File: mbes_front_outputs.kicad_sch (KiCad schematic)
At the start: 41 parts, among them IC1 BDX34C, IC2 BDX34C, IC3 BDX34C, IC4 BDX34C, Q1 D45VH10, Q10 BC337, Q2 D45VH10, Q3 BC337, Q4 BC337, Q5 BC337, Q6 BC337, Q7 BC337, Q8 BC337, Q9 BC337

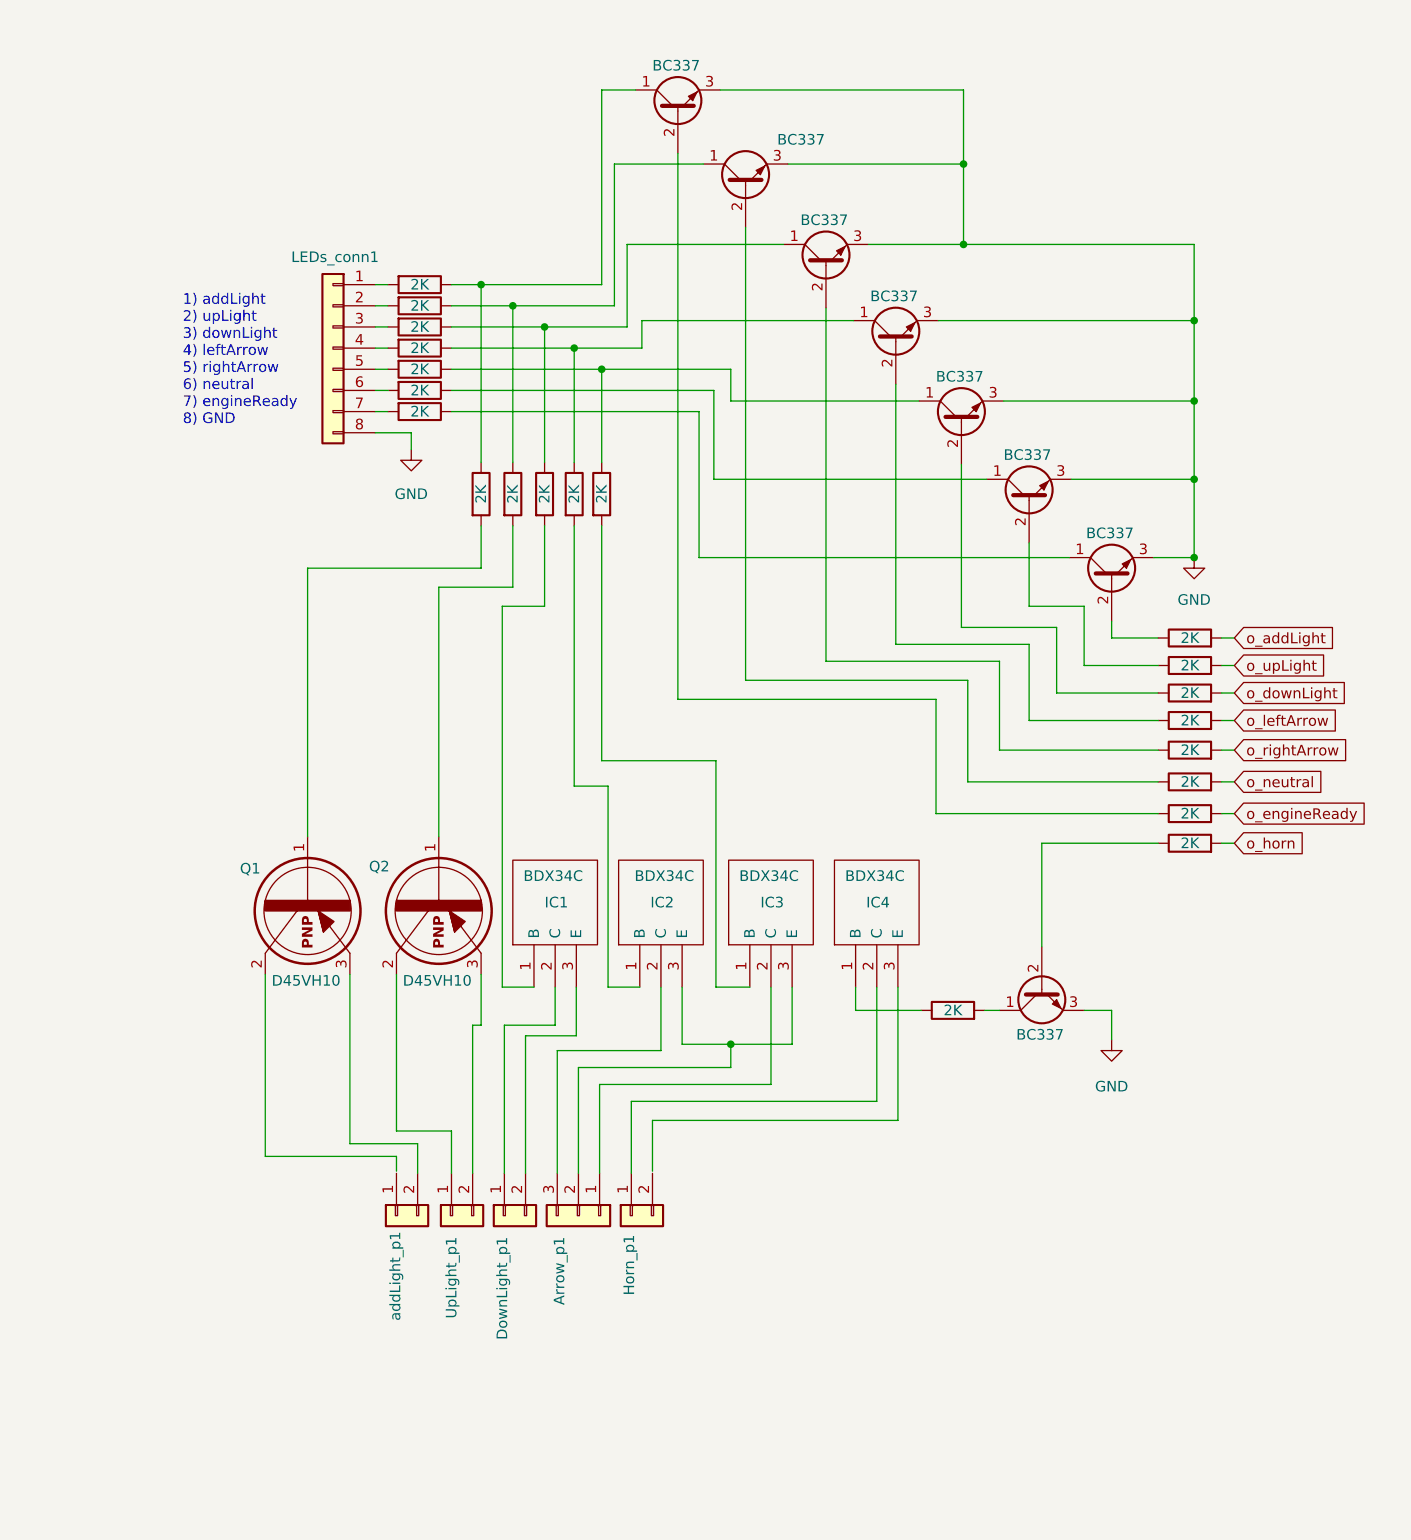
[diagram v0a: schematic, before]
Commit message: First release of all-in-one solution
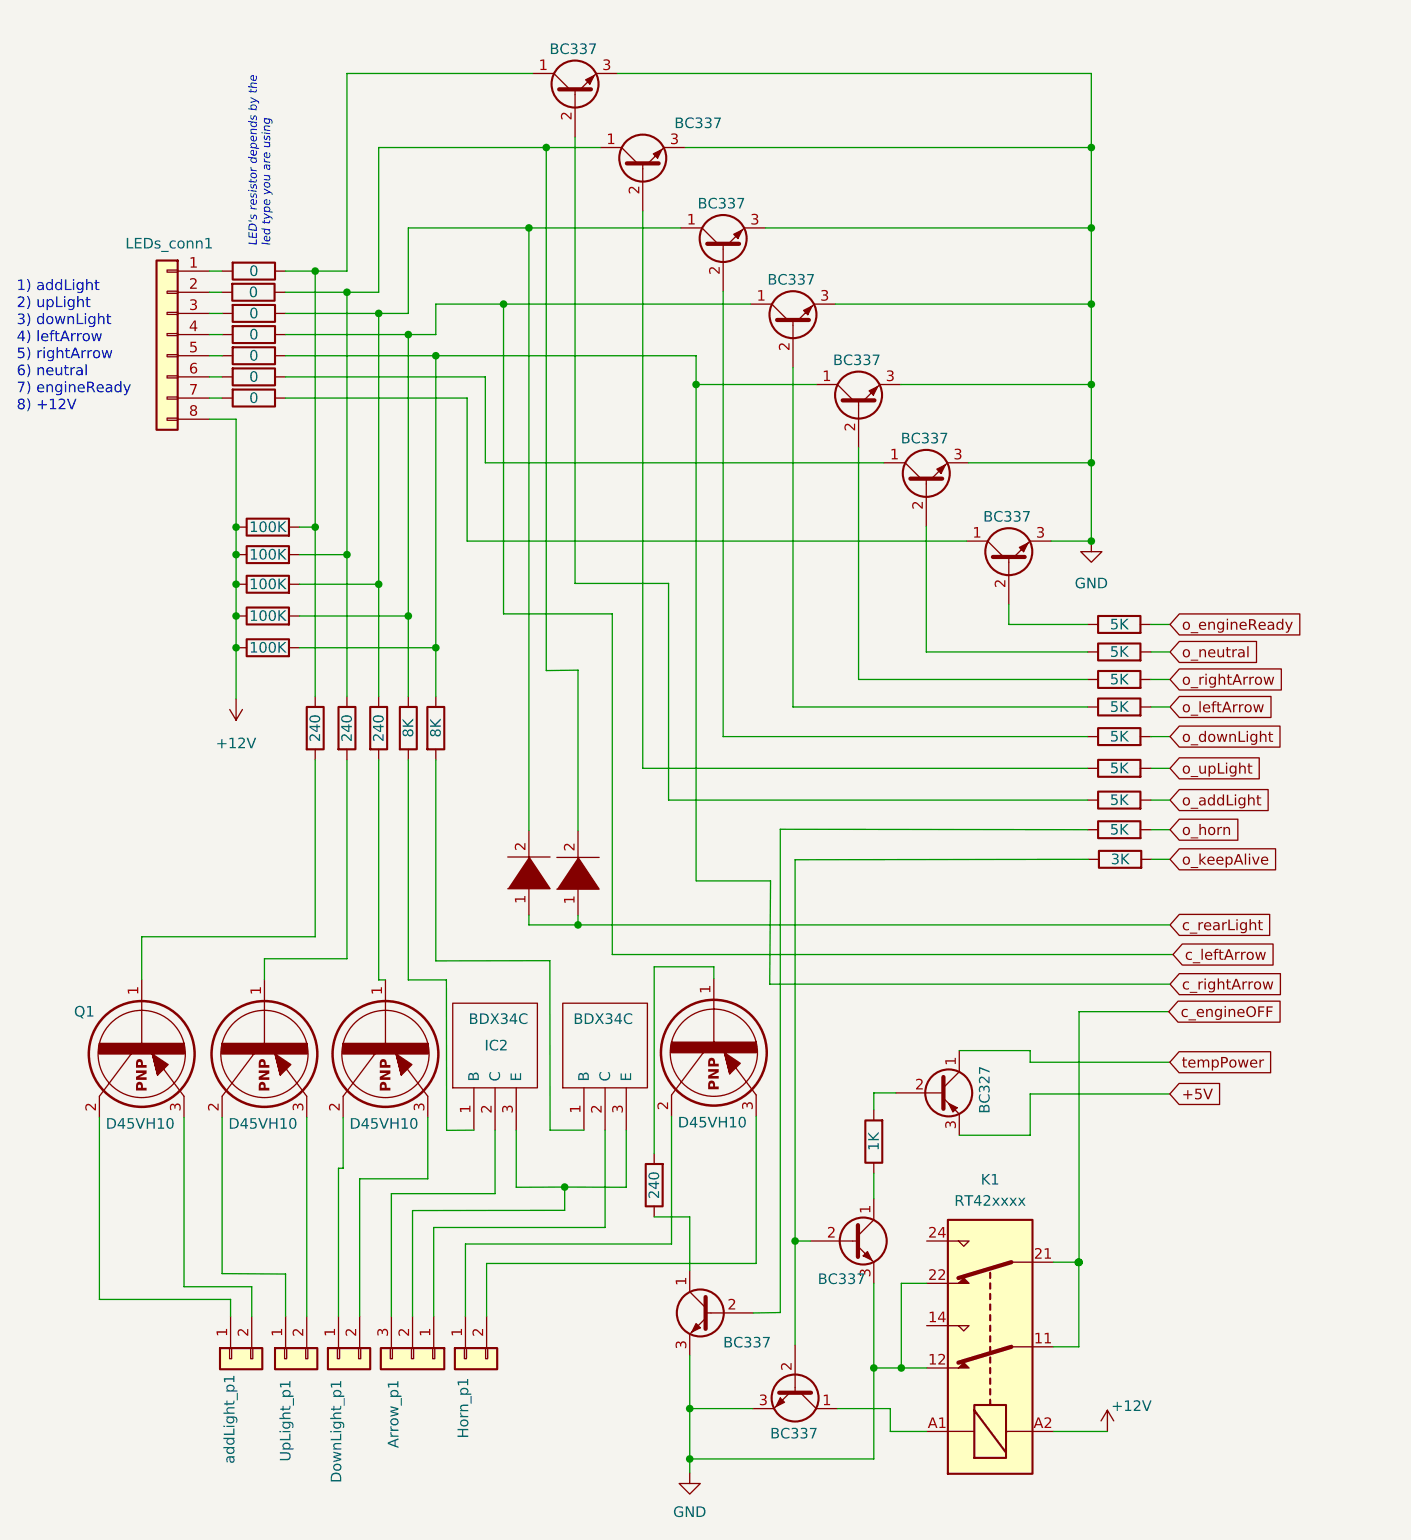
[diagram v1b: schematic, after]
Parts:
- removed IC1, IC4: BDX34C, BDX34C:TO270P460X1020X2008-3P, symbol BDX34C:BDX34C
- added D1, D2: DIODE, Diode_THT:D_DO-34_SOD68_P7.62mm_Horizontal, symbol pspice:DIODE
- added K1: RT42xxxx, Relay_THT:Relay_DPDT_Schrack-RT2-FormC_RM5mm, symbol Relay:RT42xxxx
- added Q11, Q13: BC337, Package_TO_SOT_THT:TO-92L_Inline_Wide, symbol Transistor_BJT:BC337
- added Q12: BC327, Package_TO_SOT_THT:TO-92L_Inline_Wide, symbol Transistor_BJT:BC327
- added Q14, Q15: D45VH10, Package_TO_SOT_THT:TO-220-3_Vertical, symbol D45VH10:D45VH10
- added RA24, RA25, RA26, RA27, RA28: 100K, Resistor_THT:R_Axial_DIN0207_L6.3mm_D2.5mm_P7.62mm_Horizontal, symbol Device:R
- added RA7: 1K, Resistor_THT:R_Axial_DIN0207_L6.3mm_D2.5mm_P7.62mm_Horizontal, symbol Device:R
- added RA8: 3K, Resistor_THT:R_Axial_DIN0207_L6.3mm_D2.5mm_P7.62mm_Horizontal, symbol Device:R
- LEDs_conn1: footprint (none) -> Connector_PinHeader_2.54mm:PinHeader_1x08_P2.54mm_Vertical
- Q10, Q3, Q4, Q5, Q6, Q7, Q8, Q9: footprint Package_TO_SOT_THT:TO-92_Inline -> Package_TO_SOT_THT:TO-92L_Inline_Wide
- RA1, RA2, RA3, RA4, RA5, RA6, RA9: value 2K -> 0; footprint Resistor_THT:R_Axial_DIN0207_L6.3mm_D2.5mm_P7.62mm_Horizontal -> Resistor_THT:R_Axial_DIN0207_L6.3mm_D2.5mm_P10.16mm_Horizontal
- RA10, RA11, RA12: value 2K -> 240; footprint Resistor_THT:R_Axial_DIN0207_L6.3mm_D2.5mm_P7.62mm_Horizontal -> Resistor_THT:R_Axial_DIN0414_L11.9mm_D4.5mm_P15.24mm_Horizontal
- RA13, RA14: value 2K -> 8K
- RA15: value 2K -> 240
- RA16, RA17, RA18, RA19, RA20, RA21, RA22, RA23: value 2K -> 5K
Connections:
- net GND: now also K1.12, K1.22, Q11.3 (E), Q13.3 (E); no longer LEDs_conn1.8 (Pin_8)
- net o_addLight: now also RA22.2; no longer RA16.2
- net o_downLight: now also RA20.2; no longer RA18.2
- net o_engineReady: now also RA16.2; no longer RA22.2
- net o_neutral: now also RA17.2; no longer RA21.2
- net o_rightArrow: now also RA18.2; no longer RA20.2
- net o_upLight: now also RA21.2; no longer RA17.2
- net at RA15.1: now also Q9.1 (C)
- net at RA15.2: now also Q15.1; no longer Q9.1 (C)
- net at Q3.1 (C), RA1.1, RA10.1: now also RA24.2
- net at Q1.2: now also addLight_p1.1 (Pin_1)
- net c_leftArrow: now reaches Q6.1 (C), RA13.1, RA4.1
- net c_leftArrow: now also RA27.2
- net at Q4.1 (C), RA11.1, RA2.1: now also D2.2 (A), RA25.2
- net at DownLight_p1.1 (Pin_1): now also Q14.2
- net at DownLight_p1.2 (Pin_2): now also Q14.3
- net at Horn_p1.1 (Pin_1): now also Q15.2
- net at Horn_p1.2 (Pin_2): now also Q15.3
- net at Q7.1 (C), RA14.1, RA5.1: now also RA28.2
- net at RA12.2: now also Q14.1
- net at Q5.1 (C), RA12.1, RA3.1: now also D1.2 (A), RA26.2
- new net: K1.A1, Q13.1 (C)
- new net: Q11.1 (C), RA7.1
- new net: Q12.2 (B), RA7.2
- new net: Q11.2 (B), Q13.2 (B), RA8.1
- new net +12V: K1.A2, LEDs_conn1.8 (Pin_8), RA24.1, RA25.1, RA26.1, RA27.1, RA28.1
- new net +5V: Q12.3 (E)
- new net c_engineOFF: K1.11, K1.21
- new net c_rearLight: D1.1 (K), D2.1 (K)
- new net o_keepAlive: RA8.2
- new net tempPower: Q12.1 (C)
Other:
- note added: "1) addLight 2) upLight 3) downLight 4) leftArrow 5) rightArrow 6) neutral 7) engineReady 8) +12V"
- note added: "LED's resistor depends by the led type you are using"
- note removed: "1) addLight 2) upLight 3) downLight 4) leftArrow 5) rightArrow 6) neutral 7) engineReady 8) GND"
- moved on the sheet: Arrow_p1, DownLight_p1, Horn_p1, IC2, LEDs_conn1, Q1, UpLight_p1, addLight_p1
